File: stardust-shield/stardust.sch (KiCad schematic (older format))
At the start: 12 parts, among them J1 BEXUS 28V, J2 Pololu J8557, J3 Pololu J9251, J4 DS3231M, U5 DS18B20, U6 DS18B20, U8 DHT22, U9 SSCDRNN015PASA5

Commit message: add db9 models, and update footprints
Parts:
- DSUB-1, DSUB-2: footprint Connector_Dsub:DSUB-9_Male_Horizontal_P2.77x2.84mm_EdgePinOffset4.94mm_Housed_MountingHolesOffset7.48mm -> Connector_Dsub:DSUB-9_Male_Horizontal_P2.77x2.84mm_EdgePinOffset7.70mm_Housed_MountingHolesOffset9.12mm
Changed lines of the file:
@@
 encoding utf-8
 Sheet 1 1
-Title "Stardust Overview"
+Title "Stardust Main PCB"
 Date "17 March 2020"
 Rev "2020/3/14"
@@
 F 0 "DSUB-2" H 9130 5702 50  0000 L CNN
 F 1 "DB9_Male_MountingHoles" H 9130 5611 50  0000 L CNN
-F 2 "Connector_Dsub:DSUB-9_Male_Horizontal_P2.77x2.84mm_EdgePinOffset4.94mm_Housed_MountingHolesOffset7.48mm" H 8950 5700 50  0001 C CNN
+F 2 "Connector_Dsub:DSUB-9_Male_Horizontal_P2.77x2.84mm_EdgePinOffset7.70mm_Housed_MountingHolesOffset9.12mm" H 8950 5700 50  0001 C CNN
 F 3 " ~" H 8950 5700 50  0001 C CNN
 	1    8950 5700
@@
 F 0 "DSUB-1" H 9130 3352 50  0000 L CNN
 F 1 "DB9_Male_MountingHoles" H 9130 3261 50  0000 L CNN
-F 2 "Connector_Dsub:DSUB-9_Male_Horizontal_P2.77x2.84mm_EdgePinOffset4.94mm_Housed_MountingHolesOffset7.48mm" H 8950 3350 50  0001 C CNN
+F 2 "Connector_Dsub:DSUB-9_Male_Horizontal_P2.77x2.84mm_EdgePinOffset7.70mm_Housed_MountingHolesOffset9.12mm" H 8950 3350 50  0001 C CNN
 F 3 " ~" H 8950 3350 50  0001 C CNN
 	1    8950 3350

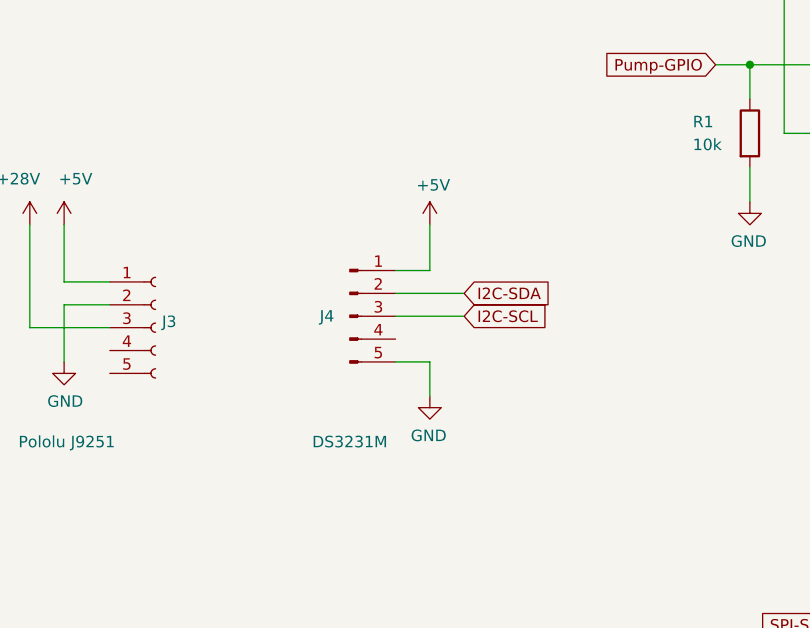
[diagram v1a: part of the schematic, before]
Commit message: rev.2 init
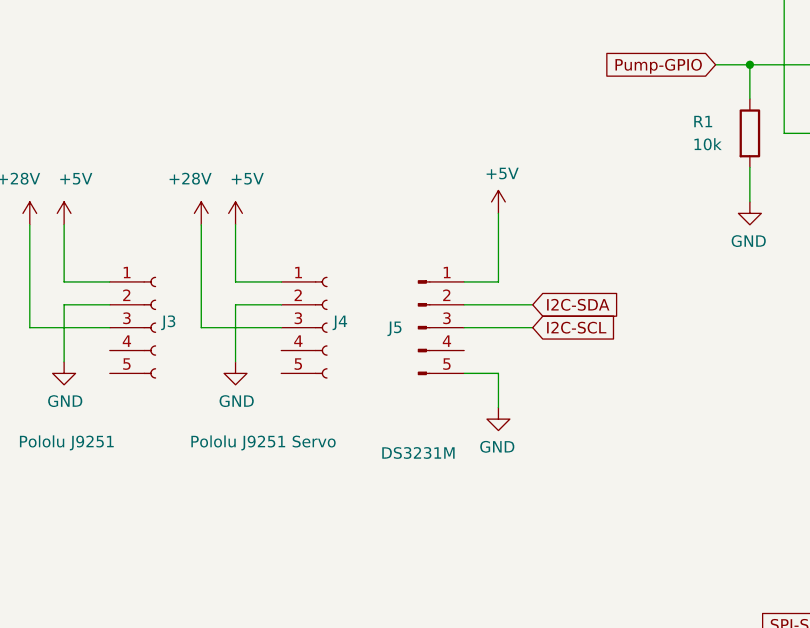
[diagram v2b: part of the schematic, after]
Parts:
- added J4: Pololu J9251 Servo, Connector_PinSocket_2.54mm:PinSocket_1x05_P2.54mm_Vertical, symbol Connector:Conn_01x05_Female
- renumbered J4 to J5
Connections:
- net +28V: now also J4.3 (Pin_3)
- net +5V: now also J4.1 (Pin_1)
- net GND: now also J4.2 (Pin_2)
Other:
- moved on the sheet: J5
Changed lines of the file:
@@
 $EndDescr
 Wire Wire Line
-	6350 4350 6650 4350
+	6650 4400 6950 4400
 Text GLabel 4800 8500 2    50   Input ~ 0
 1Wire-3
@@
 Text GLabel 4800 9700 2    50   Input ~ 0
 DHT22-3
-Text GLabel 6650 4350 2    50   Input ~ 0
+Text GLabel 6950 4400 2    50   Input ~ 0
 I2C-SDA
 $Comp
@@
 L power:+5V #PWR0134
 U 1 1 5ED92911
-P 6500 4050
-F 0 "#PWR0134" H 6500 3900 50  0001 C CNN
-F 1 "+5V" H 6515 4223 50  0000 C CNN
-F 2 "" H 6500 4050 50  0001 C CNN
-F 3 "" H 6500 4050 50  0001 C CNN
-	1    6500 4050
-	1    0    0    -1
-$EndComp
-$Comp
-L power:GND #PWR0124
-U 1 1 5E955680
-P 6500 4800
-F 0 "#PWR0124" H 6500 4550 50  0001 C CNN
-F 1 "GND" H 6505 4627 50  0000 C CNN
-F 2 "" H 6500 4800 50  0001 C CNN
-F 3 "" H 6500 4800 50  0001 C CNN
-	1    6500 4800
-	-1   0    0    -1
-$EndComp
-$Comp
-L Connector:Conn_01x05_Male J4
+P 6800 4000
+F 0 "#PWR0134" H 6800 3850 50  0001 C CNN
+F 1 "+5V" H 6815 4173 50  0000 C CNN
+F 2 "" H 6800 4000 50  0001 C CNN
+F 3 "" H 6800 4000 50  0001 C CNN
+	1    6800 4000
+	1    0    0    -1
+$EndComp
+$Comp
+L Connector:Conn_01x05_Male J5
 U 1 1 5EC929B6
-P 6150 4450
-F 0 "J4" H 6050 4450 50  0000 C CNN
-F 1 "DS3231M" H 6150 3900 50  0000 C CNN
-F 2 "Connector_PinHeader_2.54mm:PinHeader_1x05_P2.54mm_Vertical" H 6150 4450 50  0001 C CNN
-F 3 "~" H 6150 4450 50  0001 C CNN
-	1    6150 4450
-	1    0    0    -1
-$EndComp
-Wire Wire Line
-	6500 4800 6500 4650
-Wire Wire Line
-	6500 4650 6350 4650
-Wire Wire Line
-	6350 4250 6500 4250
-Wire Wire Line
-	6500 4250 6500 4050
-Text GLabel 6650 4450 2    50   Input ~ 0
+P 6450 4500
+F 0 "J5" H 6350 4500 50  0000 C CNN
+F 1 "DS3231M" H 6450 3950 50  0000 C CNN
+F 2 "Connector_PinHeader_2.54mm:PinHeader_1x05_P2.54mm_Vertical" H 6450 4500 50  0001 C CNN
+F 3 "~" H 6450 4500 50  0001 C CNN
+	1    6450 4500
+	1    0    0    -1
+$EndComp
+Wire Wire Line
+	6800 4700 6650 4700
+Wire Wire Line
+	6650 4300 6800 4300
+Text GLabel 6950 4500 2    50   Input ~ 0
 I2C-SCL
 Wire Wire Line
-	6350 4450 6650 4450
+	6650 4500 6950 4500
 Wire Wire Line
 	5100 4300 4900 4300
@@
 Text GLabel 9300 11500 2    50   Input ~ 0
 DHT22-2
+$Comp
+L power:+5V #PWR?
+U 1 1 5F1ECFCA
+P 5650 4050
+F 0 "#PWR?" H 5650 3900 50  0001 C CNN
+F 1 "+5V" H 5700 4250 50  0000 C CNN
+F 2 "" H 5650 4050 50  0001 C CNN
+F 3 "" H 5650 4050 50  0001 C CNN
+	1    5650 4050
+	1    0    0    -1
+$EndComp
+Wire Wire Line
+	5850 4300 5650 4300
+Wire Wire Line
+	5650 4300 5650 4050
+$Comp
+L power:GND #PWR?
+U 1 1 5F1ECFD2
+P 5650 4650
+F 0 "#PWR?" H 5650 4400 50  0001 C CNN
+F 1 "GND" H 5655 4477 50  0000 C CNN
+F 2 "" H 5650 4650 50  0001 C CNN
+F 3 "" H 5650 4650 50  0001 C CNN
+	1    5650 4650
+	1    0    0    -1
+$EndComp
+Wire Wire Line
+	5650 4650 5650 4400
+Wire Wire Line
+	5650 4400 5850 4400
+$Comp
+L Connector:Conn_01x05_Female J4
+U 1 1 5F1ECFDA
+P 6050 4500
+F 0 "J4" H 6078 4526 50  0000 L CNN
+F 1 "Pololu J9251 Servo" H 5450 4000 50  0000 L CNN
+F 2 "Connector_PinSocket_2.54mm:PinSocket_1x05_P2.54mm_Vertical" H 6050 4500 50  0001 C CNN
+F 3 "~" H 6050 4500 50  0001 C CNN
+	1    6050 4500
+	1    0    0    -1
+$EndComp
+Wire Wire Line
+	5850 4500 5500 4500
+Wire Wire Line
+	5500 4500 5500 4050
+$Comp
+L power:+28V #PWR?
+U 1 1 5F1ECFE2
+P 5500 4050
+F 0 "#PWR?" H 5500 3900 50  0001 C CNN
+F 1 "+28V" H 5450 4250 50  0000 C CNN
+F 2 "" H 5750 4100 50  0001 C CNN
+F 3 "" H 5750 4100 50  0001 C CNN
+	1    5500 4050
+	1    0    0    -1
+$EndComp
+Wire Wire Line
+	6800 4000 6800 4300
+Wire Wire Line
+	6800 4850 6800 4700
+$Comp
+L power:GND #PWR0124
+U 1 1 5E955680
+P 6800 4850
+F 0 "#PWR0124" H 6800 4600 50  0001 C CNN
+F 1 "GND" H 6805 4677 50  0000 C CNN
+F 2 "" H 6800 4850 50  0001 C CNN
+F 3 "" H 6800 4850 50  0001 C CNN
+	1    6800 4850
+	-1   0    0    -1
+$EndComp
 $EndSCHEMATC
